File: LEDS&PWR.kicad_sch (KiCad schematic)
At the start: 14 parts, among them J10 Conn_01x01, J13 Conn_01x01, J15 Conn_01x01, J16 Conn_01x01, J7 Conn_01x01, J9 Conn_01x01

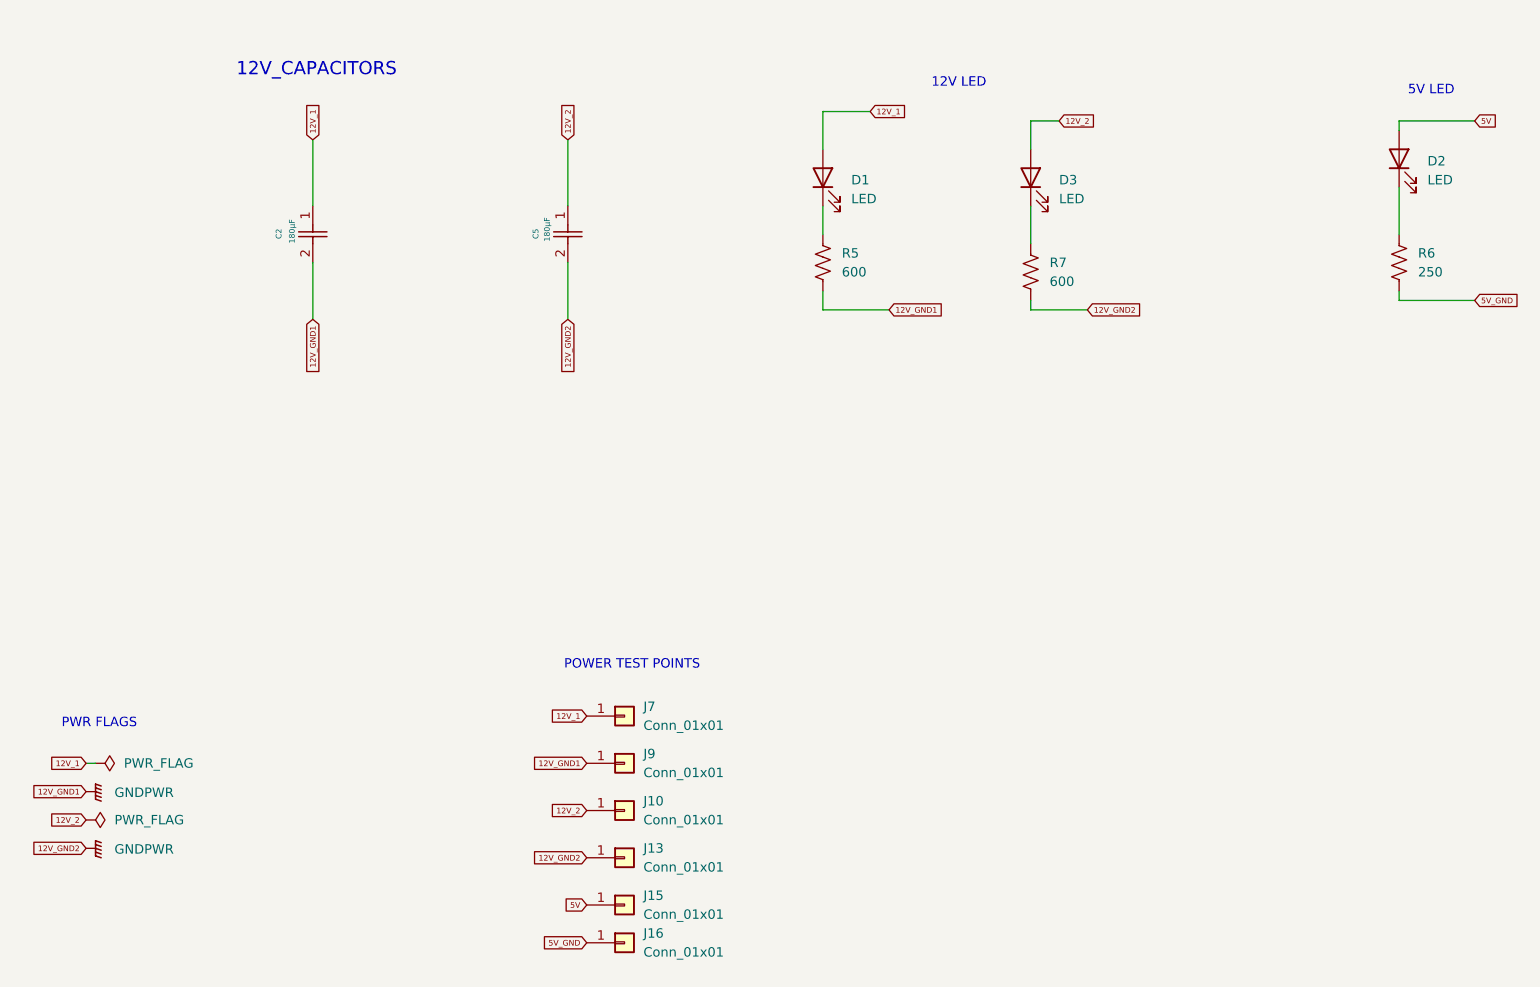
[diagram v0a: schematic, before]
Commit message: Work done on 10/23/2024
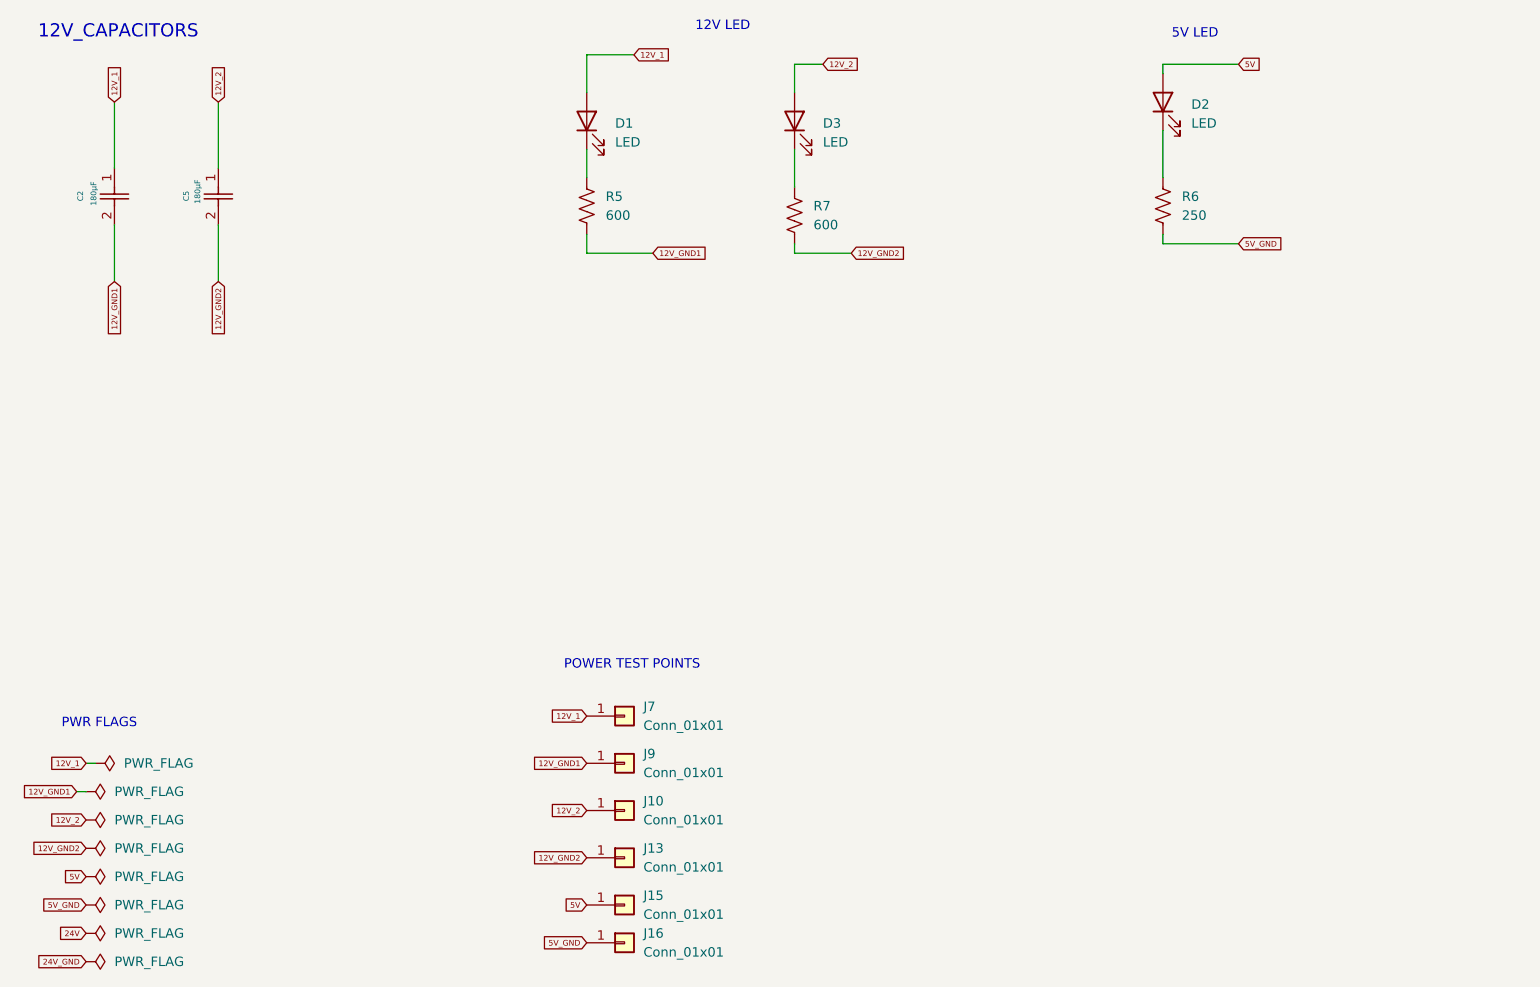
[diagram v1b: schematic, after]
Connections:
- net GNDPWR renamed 12V_GND1
- net 12V_GND1: no longer C5.2, J13.1 (Pin_1), R7.2
- new net 12V_GND2: C5.2, J13.1 (Pin_1), R7.2
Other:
- moved on the sheet: C2, C5, D1, D2, D3, R5, R6, R7
